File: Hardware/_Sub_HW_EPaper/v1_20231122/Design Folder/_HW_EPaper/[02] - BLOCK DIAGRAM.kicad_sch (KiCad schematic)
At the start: 0 parts

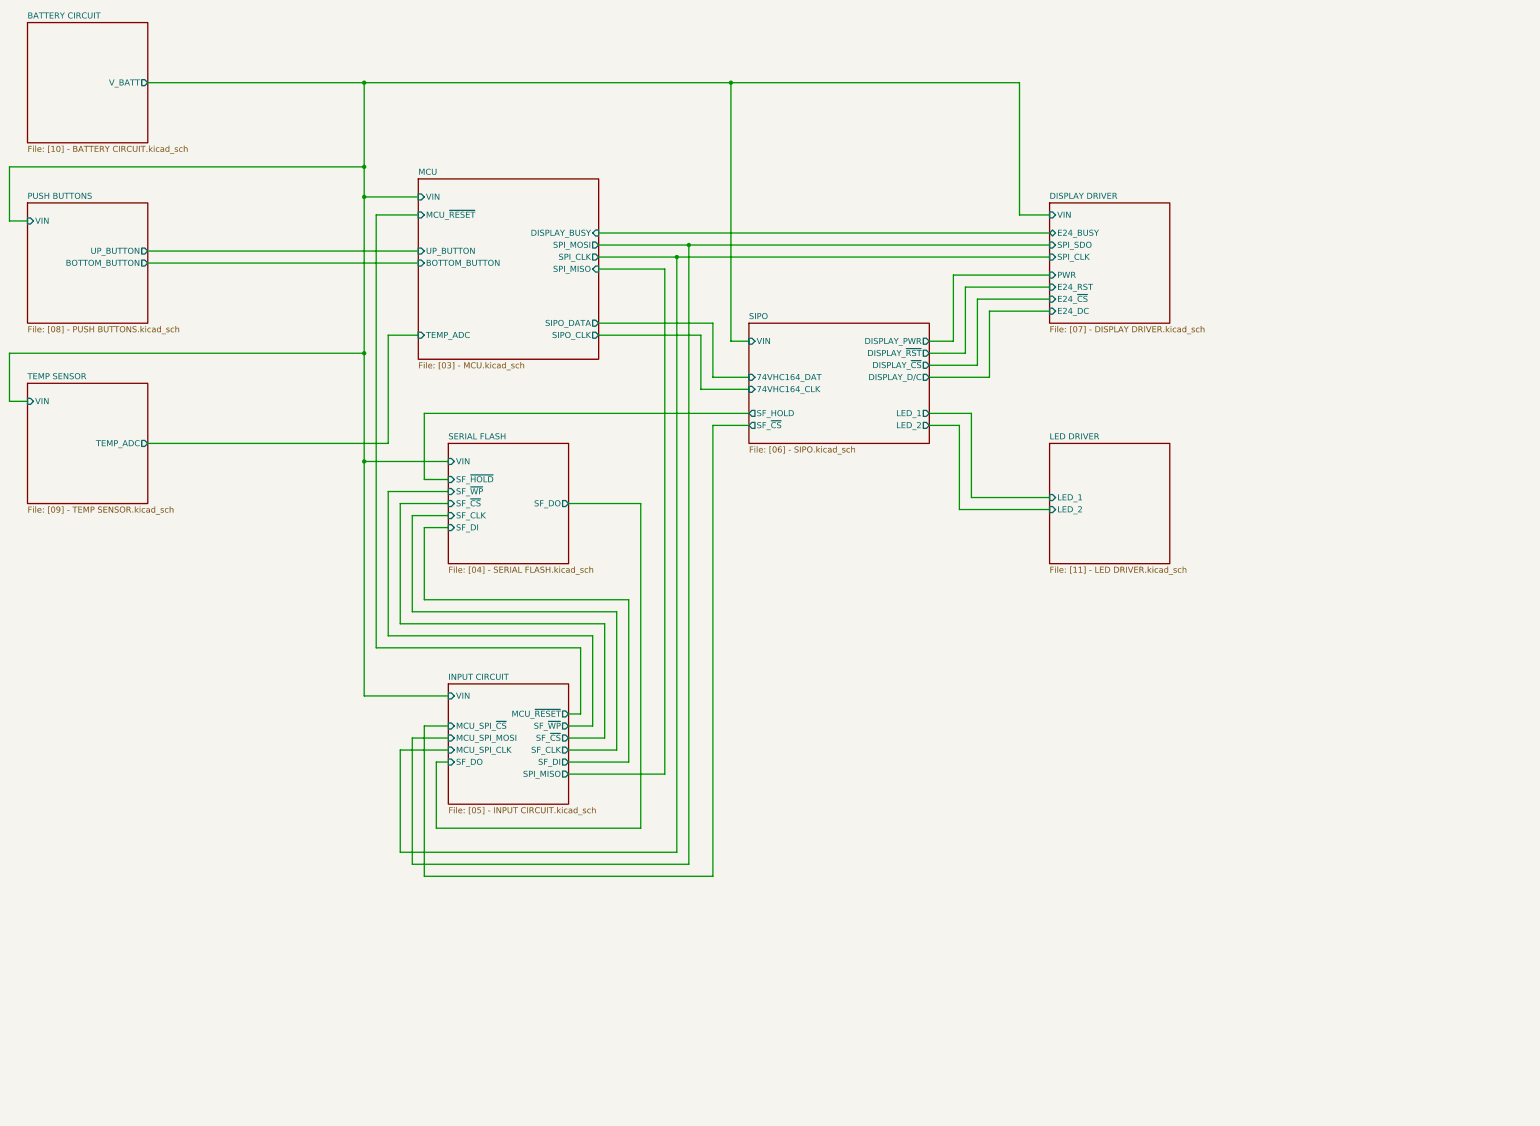
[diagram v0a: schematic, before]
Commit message: Updating file templates and structures...
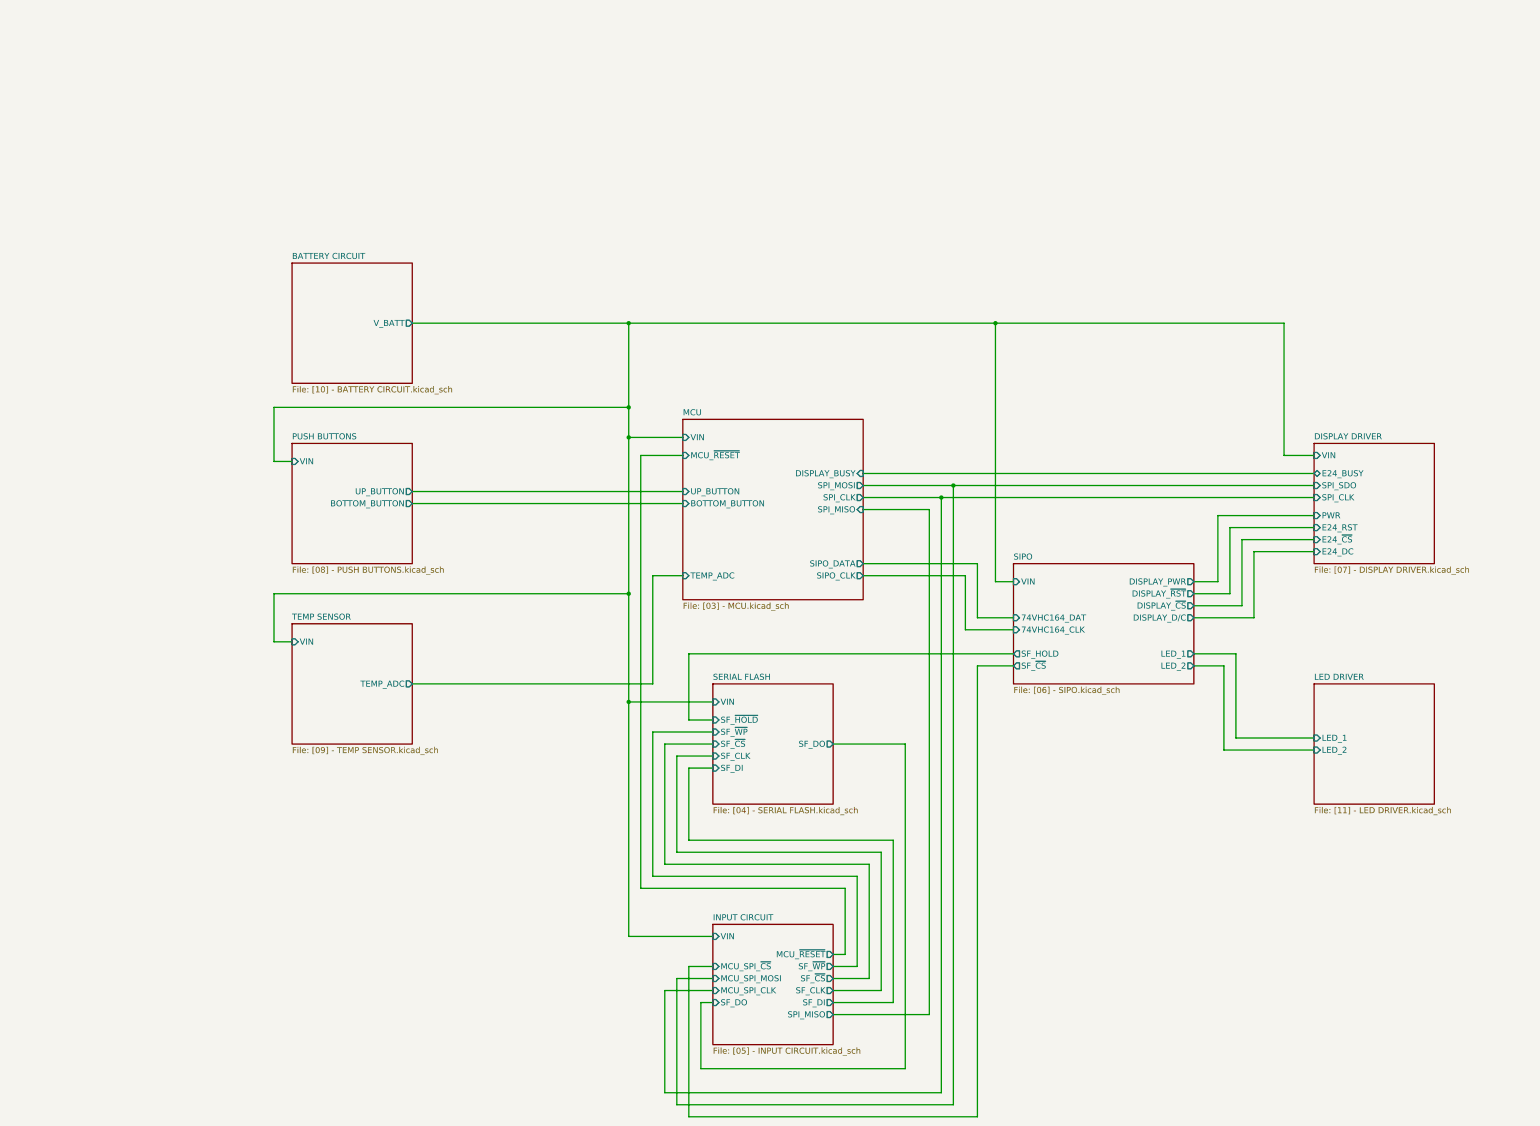
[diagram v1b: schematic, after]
